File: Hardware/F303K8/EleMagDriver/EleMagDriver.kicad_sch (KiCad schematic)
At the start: 53 parts, among them IC1 TBD62083APG, IC2 TBD62083APG, IC3 TBD62083APG, IC4 BD9E302EFJ-E2, J1 Conn_01x03_Socket, J10 RelayA, J11 RelayB, J12 RelayC, J13 RelayD, J14 RelayE, J15 RelayF, J16 RelayG, J17 RelayH, J18 RelayI, J19 RelayJ, J2 Conn_02x10_Odd_Even, J20 Floppy_Power, J21 FloppyA, J22 Floppy_Power, J23 FloppyB, J24 Floppy_Power, J25 FloppyC, J3 Barrel_Jack, J4 MotorDriverIn, J5 MotorDriveOut, J6 SolenoidA, J7 SolenoidB, J8 Jack-DC, J9 StpMotor, U1 LM3914N, U2 NUCLEO-F303K8

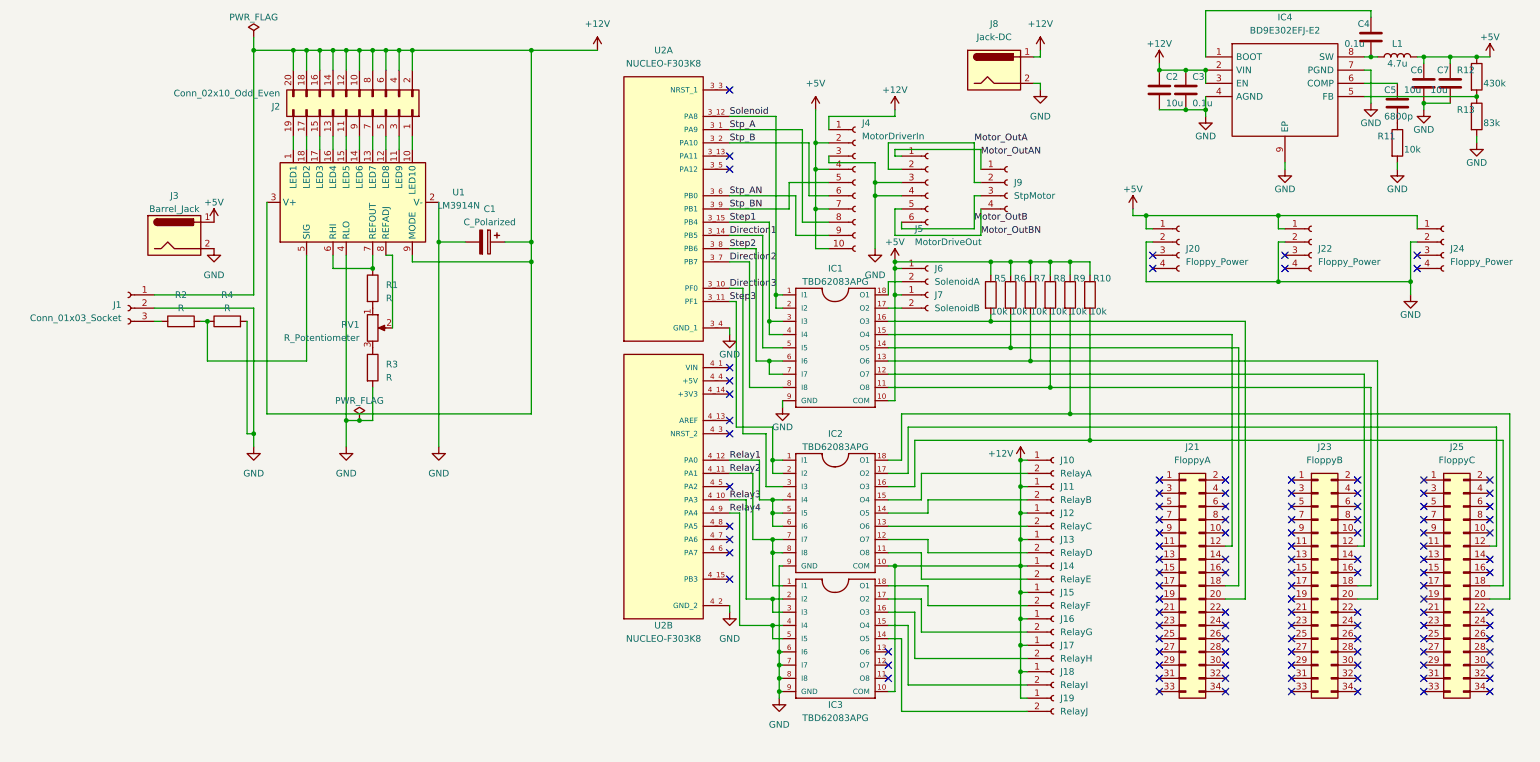
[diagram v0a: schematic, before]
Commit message: edit circuit
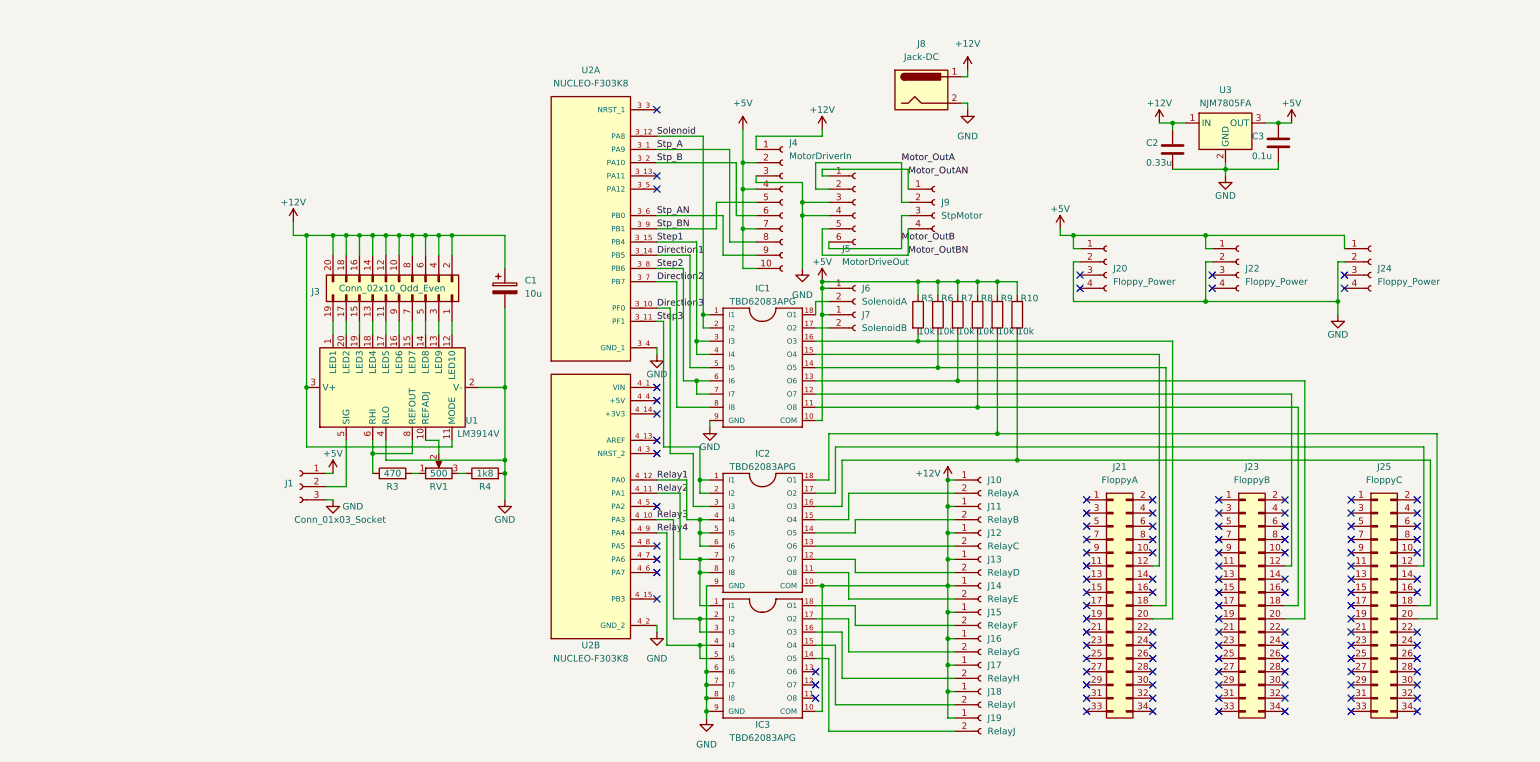
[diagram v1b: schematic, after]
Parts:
- removed C4: 0.1u, Capacitor_THT:C_Disc_D4.3mm_W1.9mm_P5.00mm, symbol Device:C
- removed C5: 6800p, Capacitor_THT:C_Disc_D4.3mm_W1.9mm_P5.00mm, symbol Device:C
- removed C6, C7: 10u, Capacitor_THT:C_Disc_D4.3mm_W1.9mm_P5.00mm, symbol Device:C
- removed IC4: BD9E302EFJ-E2, SOIC127P600X100-9N:SOIC127P600X100-9N, symbol BD9E302EFJ-E2:BD9E302EFJ-E2
- removed J3: Barrel_Jack, Connector_BarrelJack:BarrelJack_SwitchcraftConxall_RAPC10U_Horizontal, symbol Connector:Barrel_Jack
- removed L1: 4.7u, INDPM120120X800N:INDPM120120X800N, symbol Device:L
- removed R11: 10k, Resistor_THT:R_Axial_DIN0207_L6.3mm_D2.5mm_P10.16mm_Horizontal, symbol Device:R
- removed R12: 430k, Resistor_THT:R_Axial_DIN0207_L6.3mm_D2.5mm_P10.16mm_Horizontal, symbol Device:R
- removed R13: 83k, Resistor_THT:R_Axial_DIN0207_L6.3mm_D2.5mm_P10.16mm_Horizontal, symbol Device:R
- removed R2, R4: R, Resistor_SMD:R_0402_1005Metric, symbol Device:R
- removed U1: LM3914N, Package_DIP:DIP-18_W7.62mm, symbol Driver_LED:LM3914N
- added U1: LM3914V, Package_LCC:PLCC-20, symbol Driver_LED:LM3914V
- added U3: NJM7805FA, Converter_DCDC:Converter_DCDC_Murata_OKI-78SR_Vertical, symbol Converter_DCDC:OKI-78SR-3.3_1.5-W36-C
- C1: value C_Polarized -> 10u
- C2: value 10u -> 0.33u; footprint Capacitor_THT:C_Disc_D4.3mm_W1.9mm_P5.00mm -> (none)
- C3: footprint Capacitor_THT:C_Disc_D4.3mm_W1.9mm_P5.00mm -> (none)
- J3: renamed from J2; footprint Connector_PinSocket_2.00mm:PinSocket_2x10_P2.00mm_Vertical -> Connector_PinSocket_2.00mm:PinSocket_2x10_P2.00mm_Horizontal
- R3: renamed from R1; value R -> 470
- R4: renamed from R3; value R -> 1k8
- RV1: value R_Potentiometer -> 500
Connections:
- net +12V: now also U1.11 (MODE), U1.3 (V+), U3.1 (IN); no longer C3.1, J1.1 (Pin_1)
- net +5V: now also C3.1, J1.1 (Pin_1), U3.3 (OUT)
- net GND: now also J1.3 (Pin_3), U1.2 (V-), U1.4 (RLO), U3.2 (GND); no longer J1.2 (Pin_2)
- net at RV1.2: now also U1.10 (REFADJ)
- net at J3.19 (Pin_19): now also U1.1 (LED1)
- net at J3.1 (Pin_1): now also U1.12 (LED10)
- net at J3.3 (Pin_3): now also U1.13 (LED9)
- net at J3.5 (Pin_5): now also U1.14 (LED8)
- net at J3.7 (Pin_7): now also U1.15 (LED7)
- net at J3.9 (Pin_9): now also U1.16 (LED6)
- net at J3.11 (Pin_11): now also U1.17 (LED5)
- net at J3.13 (Pin_13): now also U1.18 (LED4)
- net at J3.15 (Pin_15): now also U1.19 (LED3)
- net at J3.17 (Pin_17): now also U1.20 (LED2)
- net at R3.1: now also U1.6 (RHI), U1.8 (REFOUT)
- new net: J1.2 (Pin_2), U1.5 (SIG)
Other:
- moved on the sheet: C1, IC1, IC2, IC3, J1, J10, J11, J12, J13, J14, J15, J16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

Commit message: edit circuit
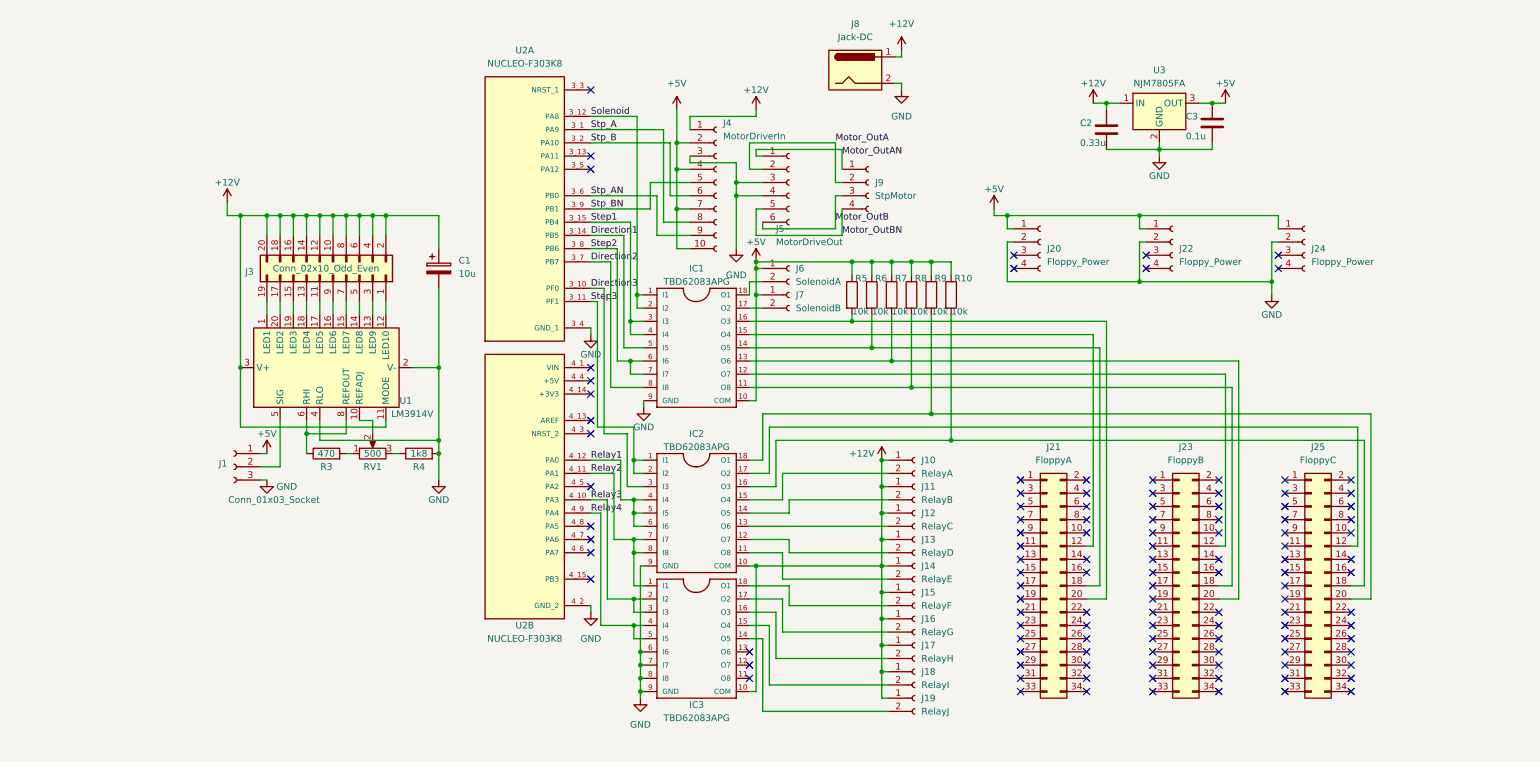
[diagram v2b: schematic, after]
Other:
- moved on the sheet: C1, C2, C3, IC1, IC2, IC3, J1, J10, J11, J12, J13, J14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

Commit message: add guitar and more
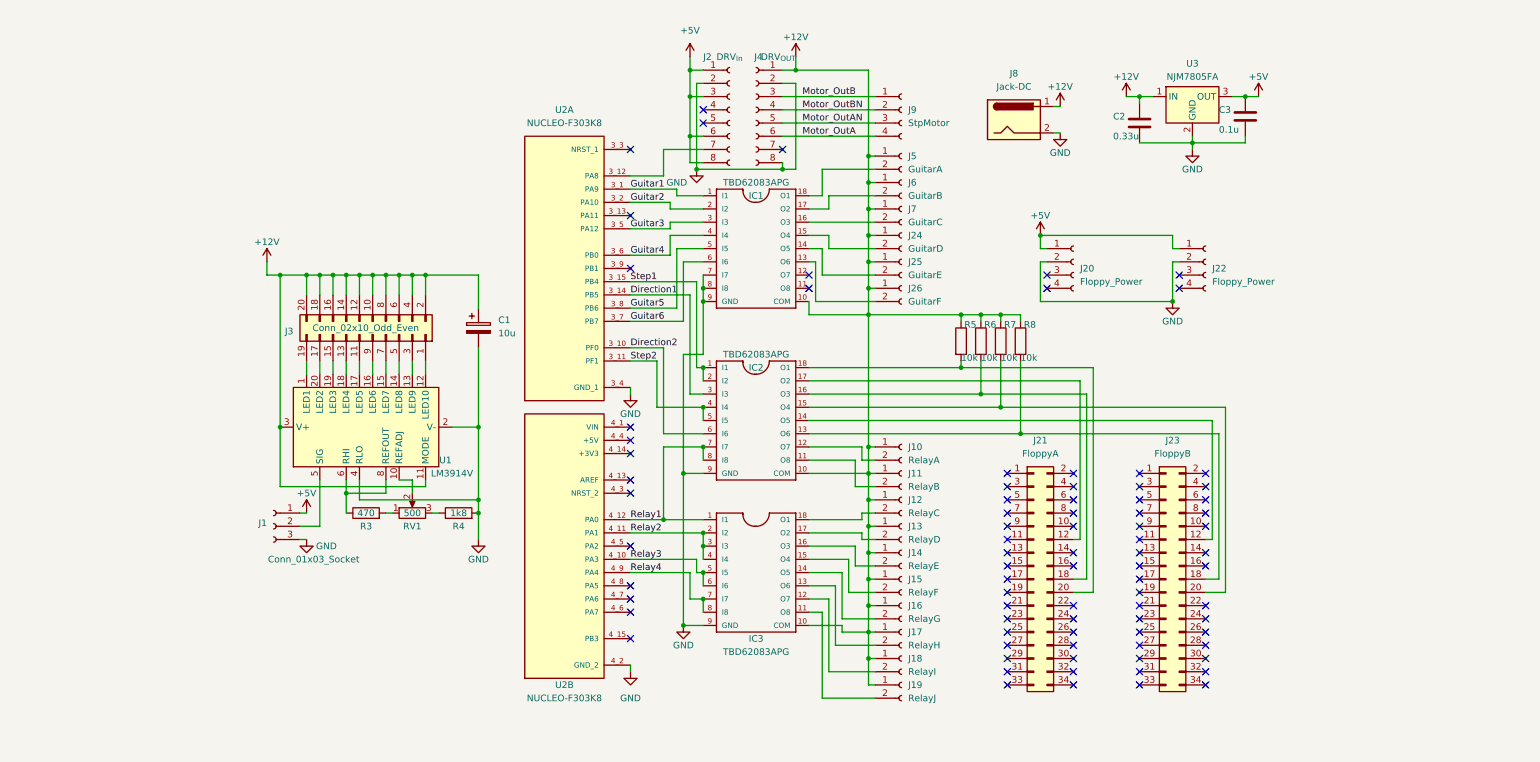
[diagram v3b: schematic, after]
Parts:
- removed J24: Floppy_Power, Connector_PinHeader_2.54mm:PinHeader_1x04_P2.54mm_Vertical, symbol Connector:Conn_01x04_Female
- removed J25: FloppyC, SHDR34W70P254_2X17_5050X820X900P:SHDR34W70P254_2X17_5050X820X900P, symbol Connector_Generic:Conn_02x17_Odd_Even
- removed J4: MotorDriverIn, Connector_PinHeader_2.54mm:PinHeader_1x10_P2.54mm_Vertical, symbol Connector:Conn_01x10_Female
- removed J5: MotorDriveOut, Connector_PinHeader_2.54mm:PinHeader_1x06_P2.54mm_Vertical, symbol Connector:Conn_01x06_Female
- removed R10, R9: 10k, Resistor_THT:R_Axial_DIN0207_L6.3mm_D2.5mm_P10.16mm_Horizontal, symbol Device:R
- added J2: DRV_{In}, symbol Connector:Conn_01x08_Socket
- added J24: GuitarD, JST_B2B-XH-A(LF)(SN):JST_B2B-XH-A(LF)(SN), symbol Connector:Conn_01x02_Female
- added J25: GuitarE, JST_B2B-XH-A(LF)(SN):JST_B2B-XH-A(LF)(SN), symbol Connector:Conn_01x02_Female
- added J26: GuitarF, JST_B2B-XH-A(LF)(SN):JST_B2B-XH-A(LF)(SN), symbol Connector:Conn_01x02_Female
- added J4: DRV_{OUT}, symbol Connector:Conn_01x08_Socket
- added J5: GuitarA, JST_B2B-XH-A(LF)(SN):JST_B2B-XH-A(LF)(SN), symbol Connector:Conn_01x02_Female
- J6: value SolenoidA -> GuitarB
- J7: value SolenoidB -> GuitarC
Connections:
- net +12V: now also IC1.10 (COM), J6.1 (Pin_1), J7.1 (Pin_1), R5.1, R6.1, R7.1, R8.1, J24.1 (Pin_1), J25.1 (Pin_1), J26.1 (Pin_1), J4.1 (Pin_1), J5.1 (Pin_1)
- net +5V: now also J2.1 (Pin_1), J2.3 (Pin_3), J2.6 (Pin_6), J2.8 (Pin_8); no longer IC1.10 (COM), J6.1 (Pin_1), J7.1 (Pin_1), R5.1, R6.1, R7.1, R8.1
- net Direction1: now also IC2.3 (I3); no longer IC1.5 (I5)
- net Direction2: now also IC2.6 (I6), U2.3_10 (PF0); no longer IC1.8 (I8), U2.3_7 (PB7)
- net GND: now also IC1.7 (I7), IC1.8 (I8), J2.2 (Pin_2), J4.2 (Pin_2), J4.8 (Pin_8); no longer IC3.6 (I6), IC3.7 (I7), IC3.8 (I8)
- net Motor_OutA: now also J9.4 (Pin_4), J4.6 (Pin_6); no longer J9.2 (Pin_2)
- net Motor_OutAN: now also J9.3 (Pin_3), J4.5 (Pin_5); no longer J9.1 (Pin_1)
- net Motor_OutB: now also J9.1 (Pin_1), J4.3 (Pin_3); no longer J9.3 (Pin_3)
- net Motor_OutBN: now also J9.2 (Pin_2), J4.4 (Pin_4); no longer J9.4 (Pin_4)
- net Relay1: now also IC2.7 (I7), IC2.8 (I8), IC3.1 (I1); no longer IC2.4 (I4), IC2.5 (I5), IC2.6 (I6)
- net Relay2: now also IC3.2 (I2), IC3.3 (I3), IC3.4 (I4); no longer IC2.7 (I7), IC2.8 (I8), IC3.1 (I1)
- net Relay3: now also IC3.5 (I5), IC3.6 (I6); no longer IC3.2 (I2), IC3.3 (I3)
- net Relay4: now also IC3.7 (I7), IC3.8 (I8); no longer IC3.4 (I4), IC3.5 (I5)
- net Step1: now also IC2.1 (I1), IC2.2 (I2); no longer IC1.3 (I3), IC1.4 (I4)
- net Step2: now also IC2.4 (I4), IC2.5 (I5), U2.3_11 (PF1); no longer IC1.6 (I6), IC1.7 (I7), U2.3_8 (PB6)
- net at J6.2 (Pin_2): now also IC1.17 (O2); no longer IC1.18 (O1)
- net at J10.2 (Pin_2): now also IC2.12 (O7); no longer IC2.15 (O4)
- net at J13.2 (Pin_2): now also IC3.17 (O2); no longer IC2.12 (O7)
- net at J7.2 (Pin_2): now also IC1.16 (O3); no longer IC1.17 (O2)
- net at J11.2 (Pin_2): now also IC2.11 (O8); no longer IC2.14 (O5)
- net at J23.18 (Pin_18), R8.2: now also IC2.13 (O6); no longer IC1.11 (O8)
- net at IC1.12 (O7): no longer J23.12 (Pin_12)
- net at J23.20 (Pin_20), R7.2: now also IC2.15 (O4); no longer IC1.13 (O6)
- net at J21.18 (Pin_18), R6.2: now also IC2.16 (O3); no longer IC1.14 (O5)
- net at IC1.15 (O4): now also J24.2 (Pin_2); no longer J21.12 (Pin_12)
- net at J21.20 (Pin_20), R5.2: now also IC2.18 (O1); no longer IC1.16 (O3)
- net Guitar3: now reaches U2.3_5 (PA12)
- net Guitar3: now also IC1.3 (I3)
- net at J17.2 (Pin_2): now also IC3.13 (O6); no longer IC3.16 (O3)
- net at J14.2 (Pin_2): now also IC3.16 (O3); no longer IC2.11 (O8)
- net at IC3.11 (O8): now also J19.2 (Pin_2)
- net at IC3.12 (O7): now also J18.2 (Pin_2)
- net at IC3.14 (O5): now also J16.2 (Pin_2); no longer J19.2 (Pin_2)
- net at IC3.15 (O4): now also J15.2 (Pin_2); no longer J18.2 (Pin_2)
- net at IC3.18 (O1): now also J12.2 (Pin_2); no longer J15.2 (Pin_2)
- net at IC2.17 (O2): now also J21.12 (Pin_12)
- removed net Direction3: IC2.3 (I3), U2.3_10 (PF0)
- removed net Solenoid: IC1.1 (I1), IC1.2 (I2), U2.3_12 (PA8)
- removed net Step3: IC2.1 (I1), IC2.2 (I2), U2.3_11 (PF1)
- net Stp_A renamed Guitar1
- net Guitar1: now also IC1.1 (I1)
- net Stp_AN renamed Guitar4
- net Guitar4: now also IC1.4 (I4)
- net Stp_B renamed Guitar2
- net Guitar2: now also IC1.2 (I2)
- net Stp_BN: no longer names the net of U2.3_9 (PB1)
- new net: IC1.13 (O6), J26.2 (Pin_2)
- new net: IC1.14 (O5), J25.2 (Pin_2)
- new net: IC1.18 (O1), J5.2 (Pin_2)
- new net: J2.7 (Pin_7), U2.3_12 (PA8)
- new net: IC2.14 (O5), J23.12 (Pin_12)
- new net Guitar5: IC1.5 (I5), U2.3_8 (PB6)
- new net Guitar6: IC1.6 (I6), U2.3_7 (PB7)
- no-connect marks 115 -> 84
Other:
- moved on the sheet: C1, C2, C3, IC1, IC2, IC3, J1, J10, J11, J12, J13, J14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
